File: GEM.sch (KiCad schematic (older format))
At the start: 0 parts

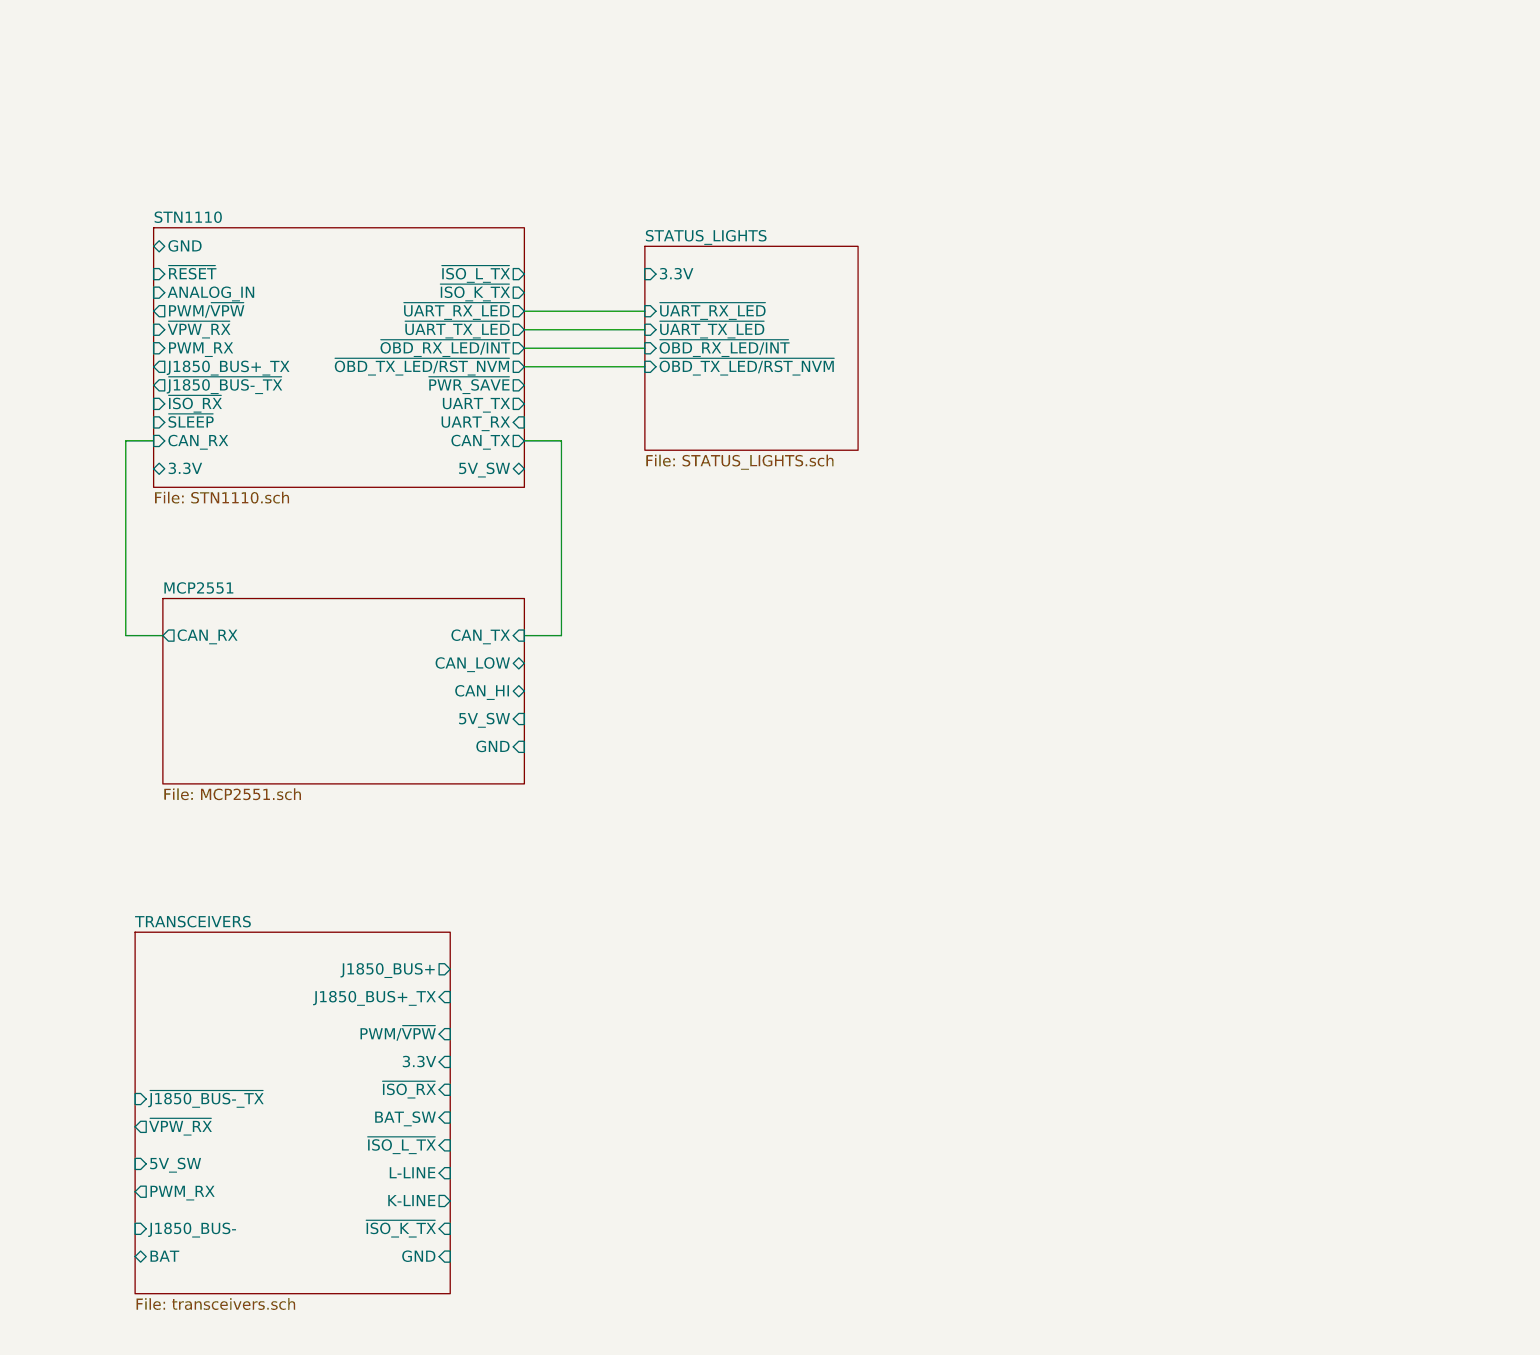
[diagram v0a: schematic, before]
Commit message: Added transceivers, power and voltage sense. Updated connections between complete sub groups with busses.
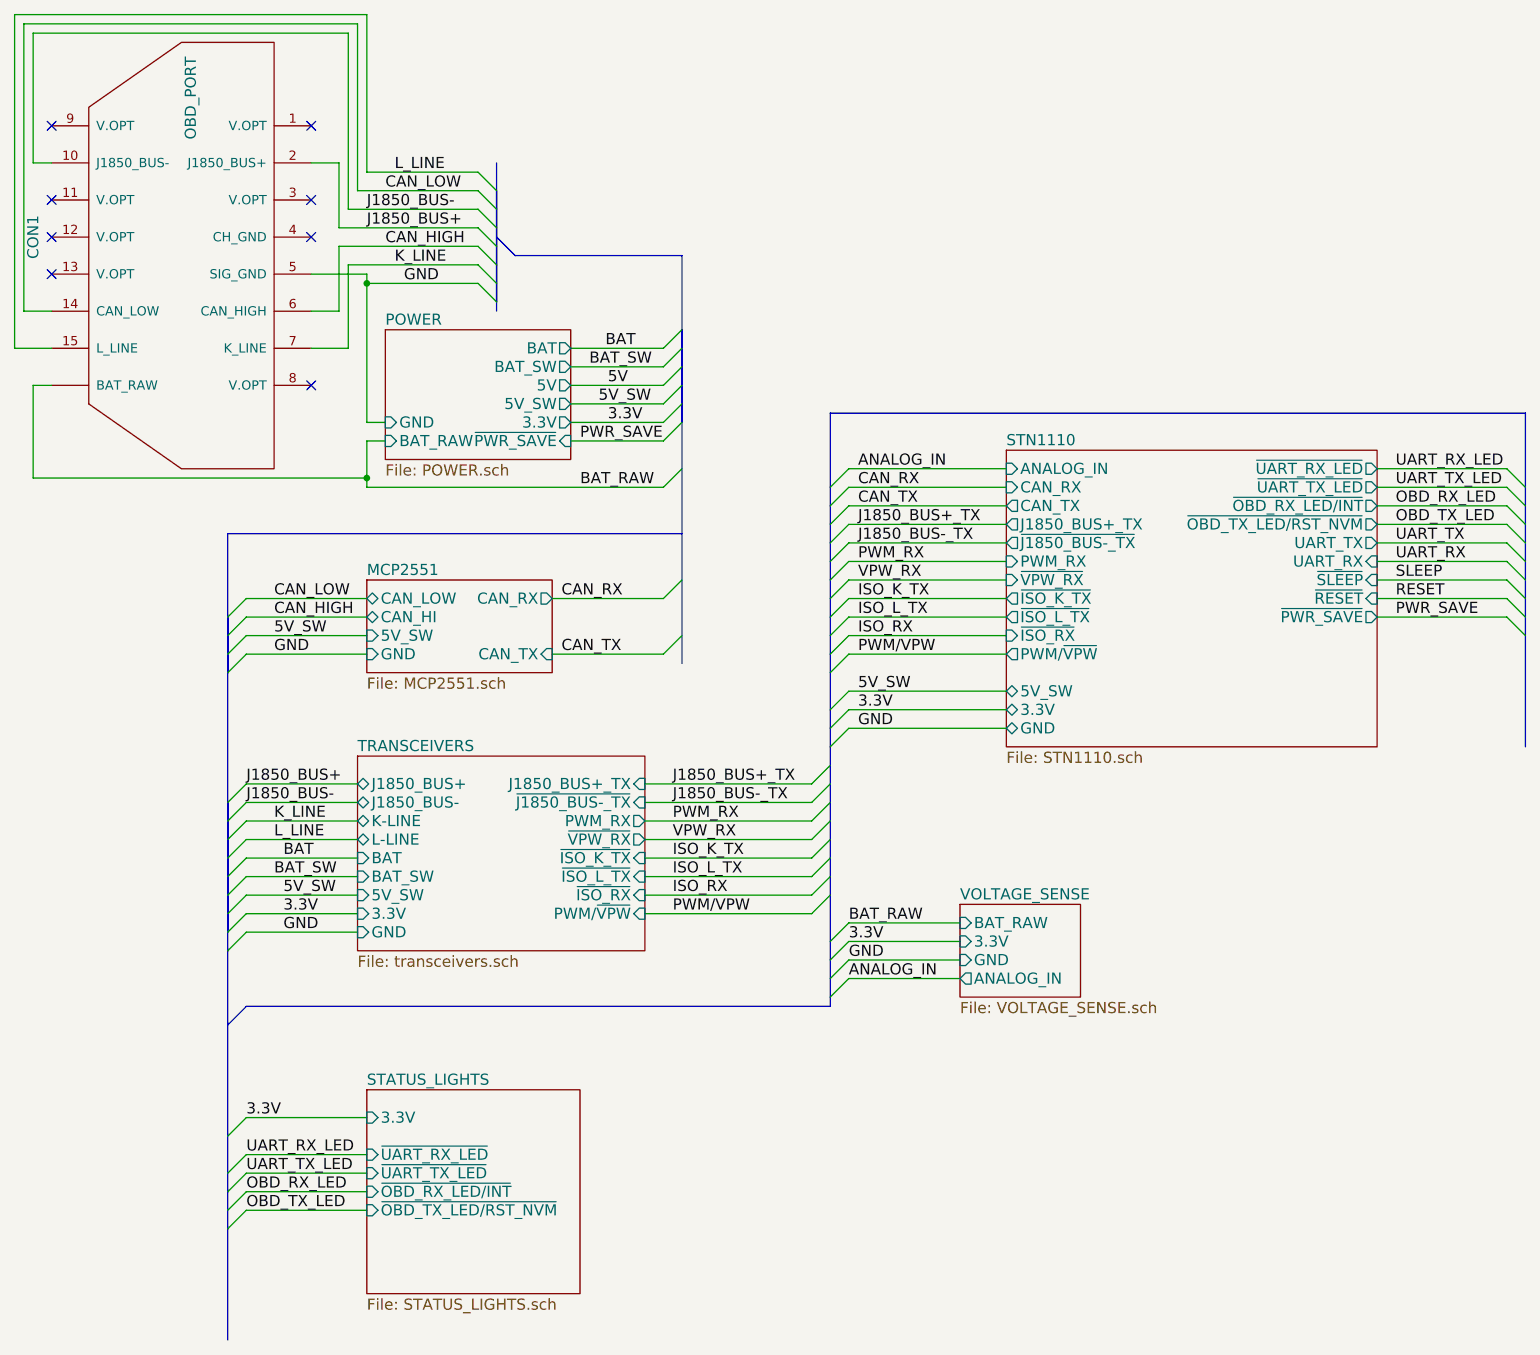
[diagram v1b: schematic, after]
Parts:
- added CON1: OBD_PORT, symbol OBD_PORT
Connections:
- new net BAT_RAW: CON1.~ (BAT_RAW)
- new net CAN_HIGH: CON1.6 (CAN_HIGH)
- new net CAN_LOW: CON1.14 (CAN_LOW)
- new net GND: CON1.5 (SIG_GND)
- new net J1850_BUS+: CON1.2 (J1850_BUS+)
- new net J1850_BUS-: CON1.10 (J1850_BUS-)
- new net K_LINE: CON1.7 (K_LINE)
- new net L_LINE: CON1.15 (L_LINE)
- no-connect marks 0 -> 8
